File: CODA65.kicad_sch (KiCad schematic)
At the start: 32 parts, among them J1 Conn_01x04, J2 Conn_01x05, U1 RP2040, U2 W25Q128JVS, U3 XC6206PxxxMR, Y1 Crystal_GND24

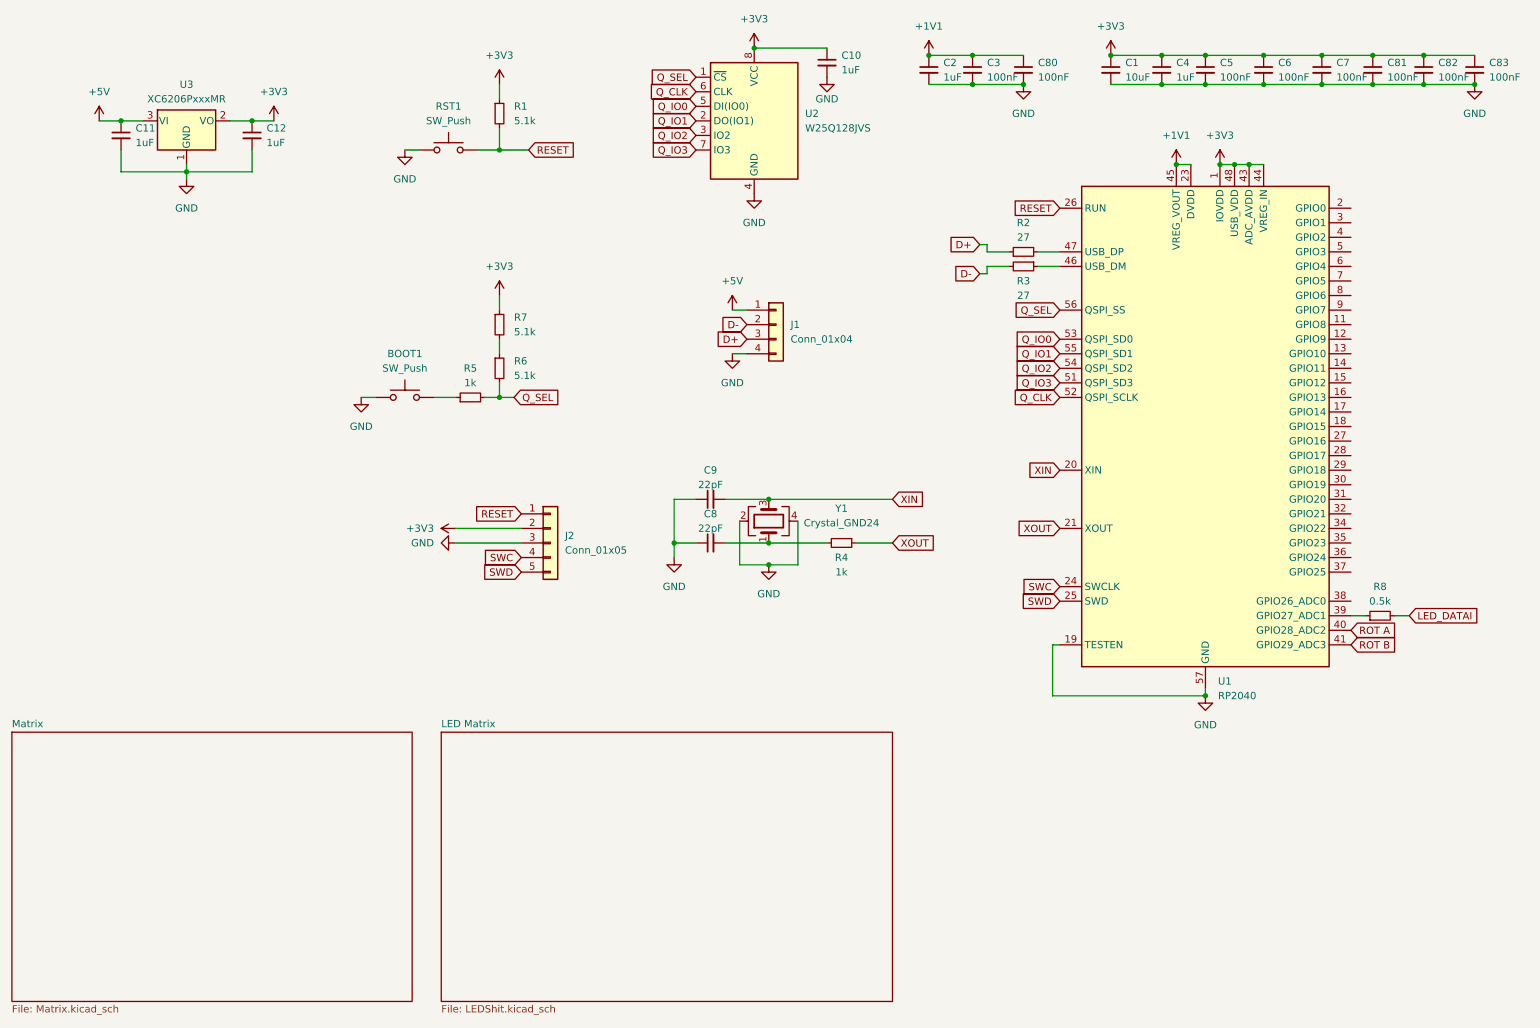
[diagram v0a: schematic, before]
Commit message: Routed more of matrix; Grounded
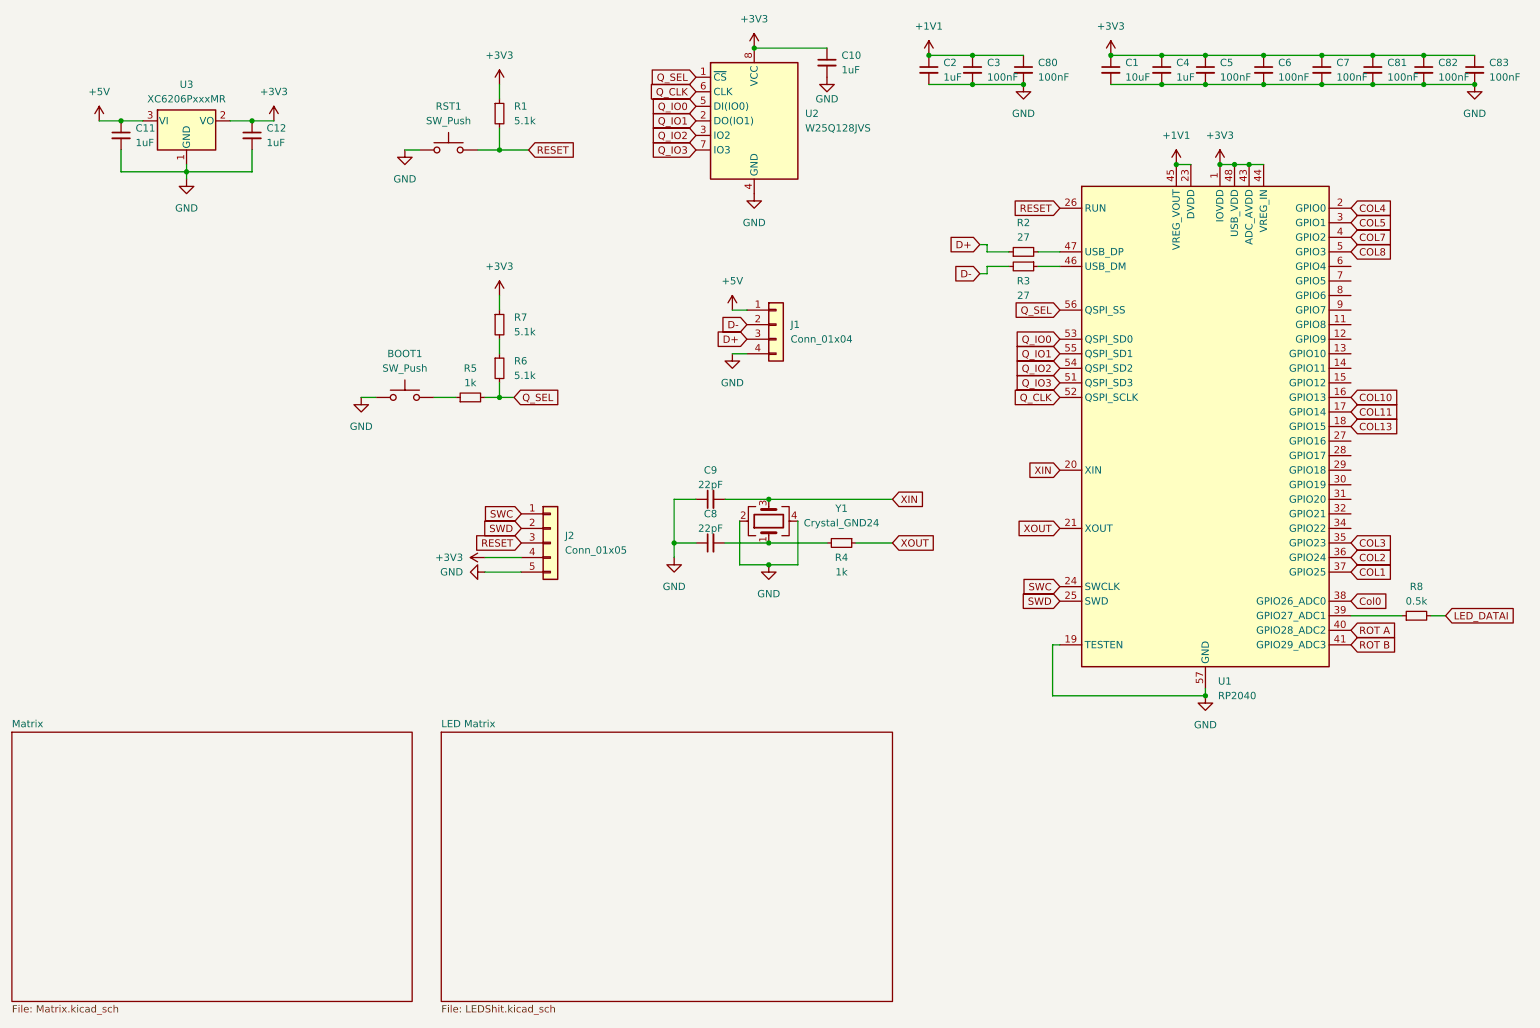
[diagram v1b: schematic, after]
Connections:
- net +3V3: now also J2.4 (Pin_4); no longer J2.2 (Pin_2)
- net GND: now also J2.5 (Pin_5); no longer J2.3 (Pin_3)
- net RESET: now also J2.3 (Pin_3); no longer J2.1 (Pin_1)
- net SWC: now also J2.1 (Pin_1); no longer J2.4 (Pin_4)
- net SWD: now also J2.2 (Pin_2); no longer J2.5 (Pin_5)
- net COL10: now reaches U1.16 (GPIO13)
- net COL11: now reaches U1.17 (GPIO14)
- net COL13: now reaches U1.18 (GPIO15)
- net COL4: now reaches U1.2 (GPIO0)
- net COL5: now reaches U1.3 (GPIO1)
- net COL3: now reaches U1.35 (GPIO23)
- net COL2: now reaches U1.36 (GPIO24)
- net COL1: now reaches U1.37 (GPIO25)
- net Col0: now reaches U1.38 (GPIO26_ADC0)
- net COL7: now reaches U1.4 (GPIO2)
- net COL8: now reaches U1.5 (GPIO3)
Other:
- moved on the sheet: R8
